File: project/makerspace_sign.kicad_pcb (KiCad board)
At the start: 2 copper layers, 76.2 x 98 mm, 24 parts, among them J1 Conn_EXT, J2 Conn_E1_M, J3 Conn_E1_F, J4 Conn_OTH_M, J5 Conn_OTH_F, J6 Conn_E2_F, J7 Conn_E2_M

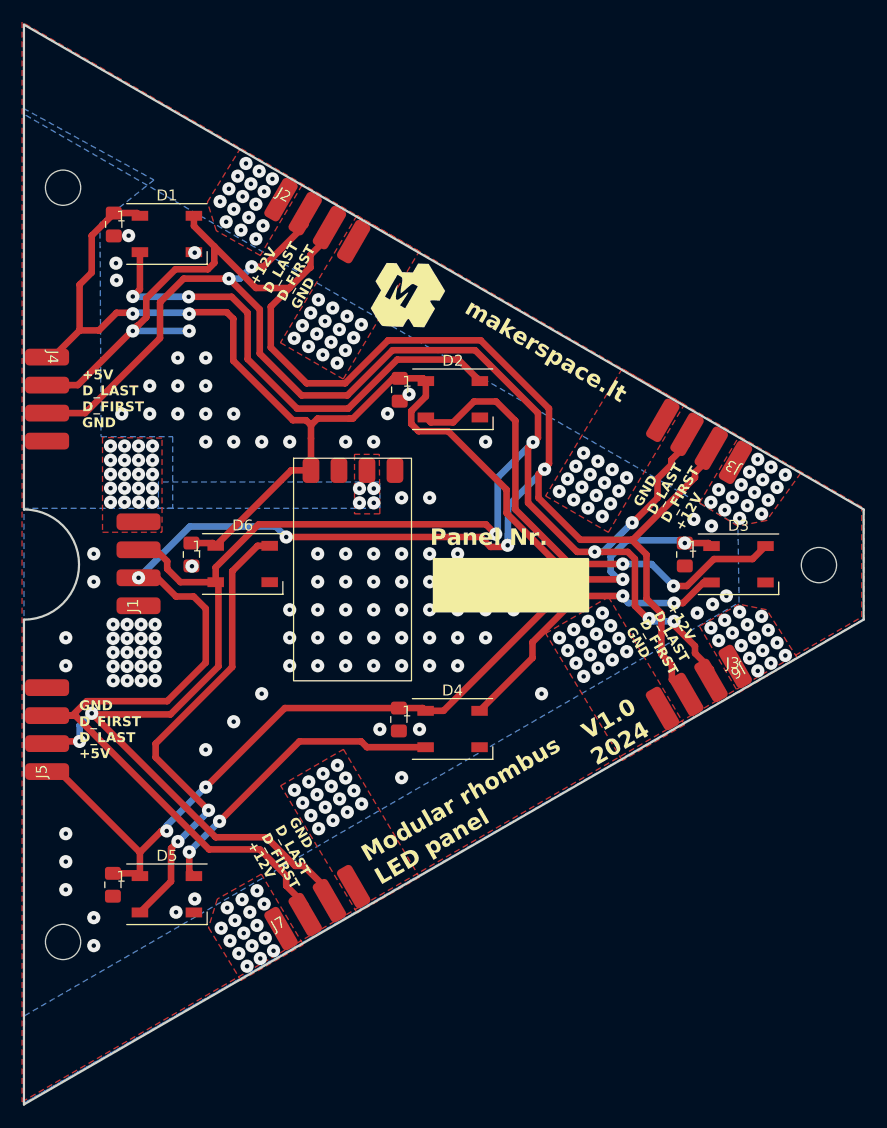
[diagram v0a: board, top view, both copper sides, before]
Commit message: 2.1
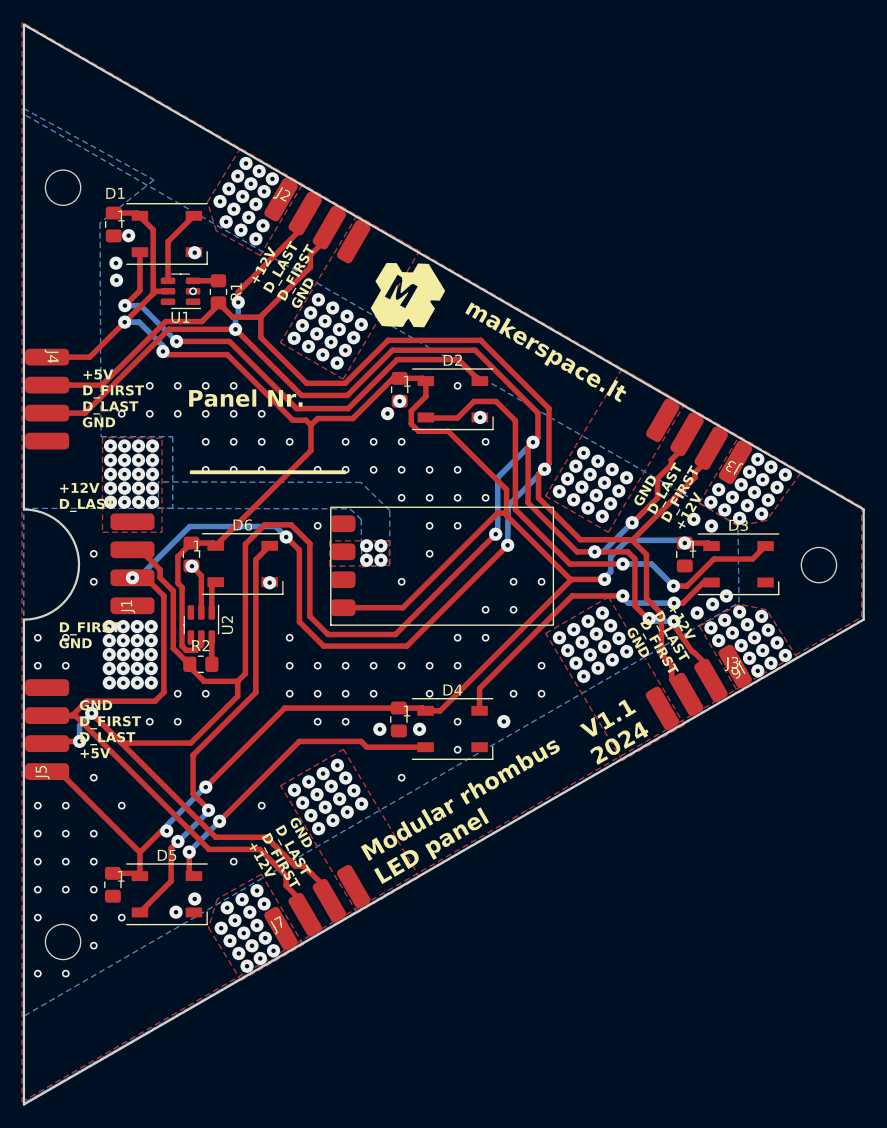
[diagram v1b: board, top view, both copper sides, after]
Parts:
- added R1: R, Resistor_SMD:R_0805_2012Metric_Pad1.20x1.40mm_HandSolder, F.Cu at (79.7, 70.7)
- added R2: R, Resistor_SMD:R_0805_2012Metric_Pad1.20x1.40mm_HandSolder, F.Cu at (78.0, 104.5)
- added U1: USBLC6-2SC6, Package_TO_SOT_SMD:SOT-23-6, F.Cu at (76.2, 70.6)
- added U2: USBLC6-2SC6, Package_TO_SOT_SMD:SOT-23-6, F.Cu at (78.1, 100.9)
- moved Buck1 15.5 mm to (89.8, 100.9), turned to 90 degrees
- moved J1 0.55 mm to (71.8, 99.1)
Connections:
- D1 pad 4: /D_FIRST -> Net-(D1-DIN)
- D6 pad 2: /D_LAST -> Net-(D6-DOUT)
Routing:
- net +5V: track 187.0 -> 212.5 mm
- net /D_LAST: track 226.0 -> 245.4 mm
- net /D_FIRST: track 236.6 -> 228.7 mm, vias 6 -> 4
- net Net-(D1-DIN): track 0.00 -> 6.87 mm
- net GND: track 0.00 -> 4.55 mm, vias 171 -> 199
- net /D_56: track 42.8 -> 39.3 mm
- net Net-(D6-DOUT): track 0.00 -> 2.89 mm
- net Net-(R2-Pad2): track 0.00 -> 2.42 mm
- net Net-(R1-Pad1): track 0.00 -> 2.30 mm
- net /D_12: track 45.1 -> 44.1 mm
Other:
- board text added: "+12V D_LAST"
- board text added: "+5V D_FIRST D_LAST GND"
- board text added: "D_FIRST GND"
- board text added: "V1.1 2024"
- board text removed: "+5V D_LAST D_FIRST GND"
- board text removed: "V1.0 2024"
